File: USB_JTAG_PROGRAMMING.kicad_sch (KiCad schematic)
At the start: 85 parts, among them J16 10118194-0001LF, U3 FT2232HQ, U36 MIC5504-3.3YM5-TR, U37 93LC56BT-I/OT, U38 KC2016K12.0000C1GE00, U39 SN74LVC1T45DBVR, U40 NC7WZ07P6X, U41 NC7SZ125M5X, U42 SN74LVC1T45DBVR, U43 SN74LVC1T45DBVR, U44 SN74LVC1T45DBVR, U45 SN74LVC1T45DBVR, U46 NC7WZ126K8X, U47 NC7WZ126K8X

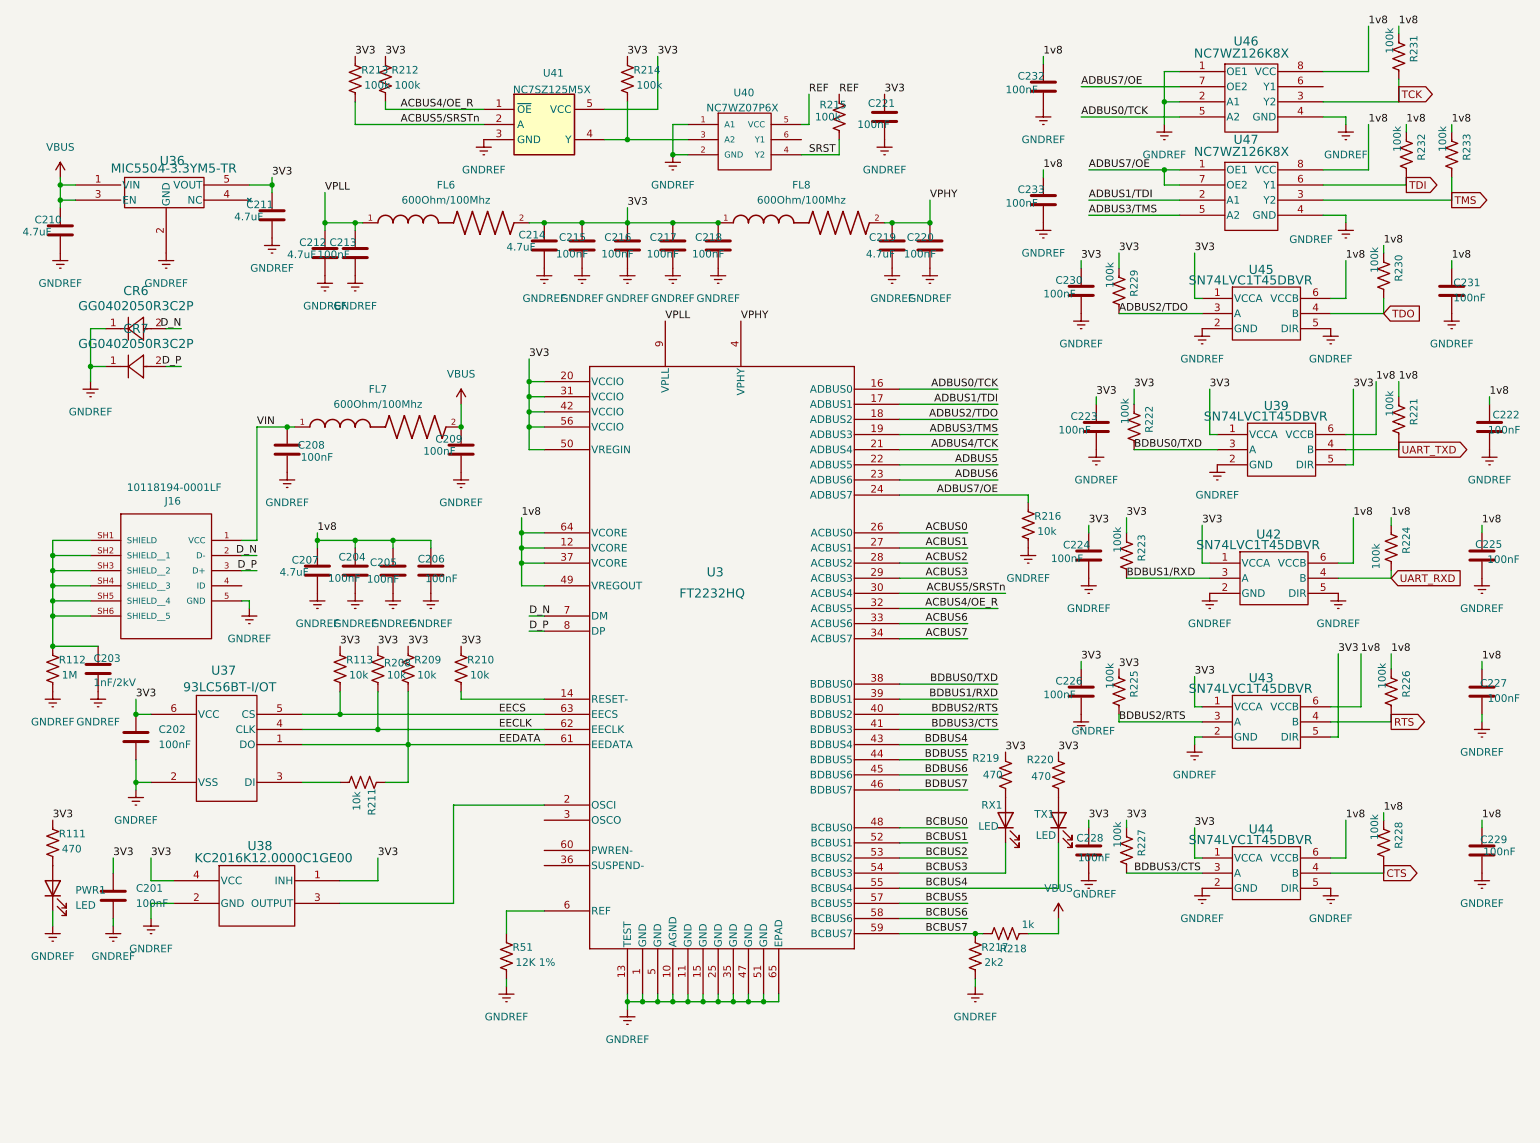
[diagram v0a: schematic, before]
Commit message: Layout update
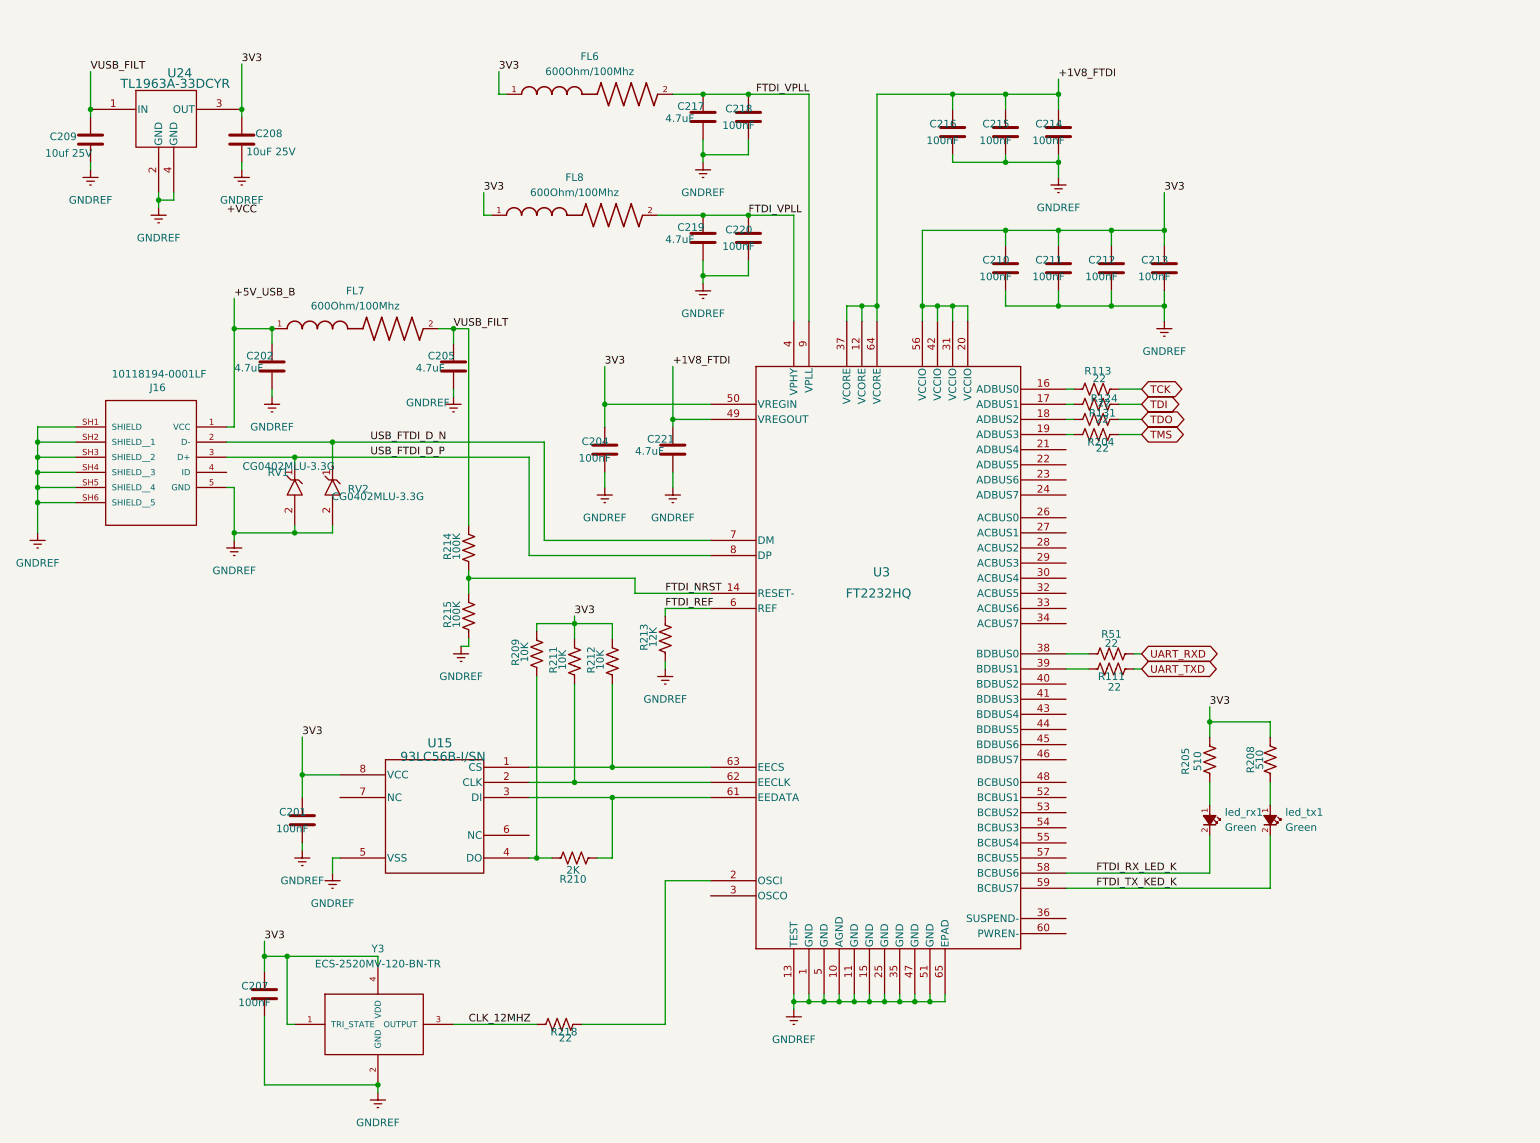
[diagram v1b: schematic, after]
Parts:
- removed C203: 1nF/2kV, footprints:C_1210_3225Metric, symbol Device:C
- removed C206, C222, C223, C224, C225, C226, C227, C228, C229, C230, C231, C232, C233: 100nF, footprints:C_0201_0603Metric, symbol Device:C
- removed CR6, CR7: GG0402050R3C2P, footprints:CR_050R3C2P_AVX, symbol GG0402050R3C2P:GG0402050R3C2P
- removed PWR1, RX1, TX1: LED, footprints:LED_0402_1005Metric, symbol Device:LED
- removed R112: 1M, footprints:R_0402, symbol Device:R_US
- removed R216: 10k, footprints:R_0402, symbol Device:R_US
- removed R217: 2k2, footprints:R_0402, symbol Device:R_US
- removed R219, R220: 470, footprints:R_0402, symbol Device:R_US
- removed R221, R222, R223, R224, R225, R226, R227, R228, R229, R230, R231, R232, R233: 100k, footprints:R_0402, symbol Device:R_US
- removed U36: MIC5504-3.3YM5-TR, footprints:SOT-23-5_MC_MCH, symbol MIC5504_3_3YM5_TR:MIC5504-3.3YM5-TR
- removed U37: 93LC56BT-I/OT, footprints:SOT-23-6_MC_MCH, symbol 93LC56BT_I_OT:93LC56BT-I_OT
- removed U38: KC2016K12.0000C1GE00, footprints:KC2016K_KYO, symbol KC2016K12-0000C1GE00:KC2016K12.0000C1GE00
- removed U39, U42, U43, U44, U45: SN74LVC1T45DBVR, footprints:DBV0006A_L, symbol SN74LVC1T45DBVR:SN74LVC1T45DBVR
- removed U40: NC7WZ07P6X, footprints:NC7WZ07P6X, symbol NC7WZ07P6X:NC7WZ07P6X
- removed U41: NC7SZ125M5X, footprints:SC-74A_318BQ_ONS, symbol 74xGxx:NC7SZ125M5X
- removed U46, U47: NC7WZ126K8X, footprints:US8-8_2P1X2P4_ONS, symbol NC7WZ126:NC7WZ126K8X
- added R124, R131, R204: 22, footprints:R_0201_0603Metric, symbol Device:R_US
- added R205: 510, footprints:R_0201_0603Metric, symbol Device:R_US
- added RV1, RV2: CG0402MLU-3.3G, footprints:VARC1005X41N, symbol CG0402MLU-3_3G:CG0402MLU-3.3G
- added U15: 93LC56B-I/SN, footprints:SOIC8-N_MC_MCH, symbol 93LC56B-I-SN:93LC56B-I_SN
- added U24: TL1963A-33DCYR, footprints:DCY4_TEX, symbol TL1963A-33DCYR:TL1963A-33DCYR
- added Y3: ECS-2520MV-120-BN-TR, footprints:OSCCC250X200X90N, symbol ECS-2520MV-120-BN-TR:ECS-2520MV-120-BN-TR
- added led_rx1, led_tx1: Green, footprints:LED_0402_1005Metric, symbol Aquiot:LED
- C202, C205, C217, C221: value 100nF -> 4.7uF; footprint footprints:C_0201_0603Metric -> footprints:C_0402; LCSC PN c1525 -> c23733
- C207, C210, C211, C212, C214: value 4.7uF -> 100nF; footprint footprints:C_0402 -> footprints:C_0201_0603Metric; LCSC PN c23733 -> c1525
- C208: value 100nF -> 10uF 25V; footprint footprints:C_0201_0603Metric -> footprints:C_0402; LCSC PN c1525 -> c23733
- C209: value 100nF -> 10uf 25V; footprint footprints:C_0201_0603Metric -> footprints:C_0402; LCSC PN c1525 -> c23733
- R111: value 470 -> 22; footprint footprints:R_0402 -> footprints:R_0201_0603Metric; LCSC PN C114877 -> (none)
- R113: value 10k -> 22; footprint footprints:R_0402 -> footprints:R_0201_0603Metric; LCSC PN C60490 -> (none)
- R208: value 10k -> 510; footprint footprints:R_0402 -> footprints:R_0201_0603Metric; LCSC PN C60490 -> (none)
- R209, R211: value 10k -> 10K; footprint footprints:R_0402 -> footprints:R_0201_0603Metric; LCSC PN C60490 -> (none)
- R210: value 10k -> 2K; footprint footprints:R_0402 -> footprints:R_0201_0603Metric; LCSC PN C60490 -> (none)
- R212: value 100k -> 10K; footprint footprints:R_0402 -> footprints:R_0201_0603Metric; LCSC PN C60491 -> (none)
- R213: value 100k -> 12K; footprint footprints:R_0402 -> footprints:R_0201_0603Metric; LCSC PN C60491 -> (none)
- R214, R215: value 100k -> 100K; footprint footprints:R_0402 -> footprints:R_0201_0603Metric; LCSC PN C60491 -> (none)
- R218: value 1k -> 22; footprint footprints:R_0402 -> footprints:R_0201_0603Metric; LCSC PN c106235 -> (none)
- R51: value 12K 1% -> 22; footprint footprints:R_0402 -> footprints:R_0201_0603Metric; LCSC PN C114760 -> (none)
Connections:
- net BDBUS0/TXD is gone; now on an unnamed net: U3.38 (BDBUS0)
- net REF is gone; now on net GNDREF: R215.1
- net 3V3: now also C204.1, C207.1, C208.1, C210.1, C212.1, C213.1, FL6.1, R208.2, R209.2, R211.2, R212.2, R205.2, U15.8 (VCC), U24.3 (OUT), Y3.1 (TRI_STATE), Y3.4 (VDD); no longer C202.1, C214.1, C215.1, C216.1, C217.1, C218.1, C221.1, FL6.2, R111.1, R113.1, R208.1, R209.1, R210.1, R212.1, R213.1, R214.1
- net GNDREF: now also J16.SH1 (SHIELD), J16.SH2 (SHIELD__1), J16.SH3 (SHIELD__2), J16.SH4 (SHIELD__3), J16.SH5 (SHIELD__4), J16.SH6 (SHIELD__5), R213.1, RV1.2, RV2.2, U15.5 (VSS), U24.2 (GND), U24.4 (GND), Y3.2 (GND); no longer R51.2
- net TCK: now also R113.2
- net TDI: now also R124.2
- net TDO: now also R131.2
- net TMS: now also R204.2
- net UART_RXD: now also R51.2
- net UART_TXD: now also R111.2
- net at R51.1: no longer U3.6 (REF)
- net at U3.2 (OSCI): now also R218.2
- net at R210.2: now also R209.1, U15.4 (DO); no longer U3.14 (RESET-)
- net VUSB_FILT: now reaches R214.2
- net VUSB_FILT: now also C205.1, C209.1, FL7.2, U24.1 (IN)
- net 1v8 renamed +1V8_FTDI
- net +1V8_FTDI: now also C214.1, C215.1, C216.1, C221.1; no longer C204.1, C205.1, C207.1
- net ACBUS0: no longer names the net of U3.26 (ACBUS0)
- net ACBUS1: no longer names the net of U3.27 (ACBUS1)
- net ACBUS2: no longer names the net of U3.28 (ACBUS2)
- net ACBUS3: no longer names the net of U3.29 (ACBUS3)
- net ACBUS4/OE_R: no longer names the net of U3.32 (ACBUS5)
- net ACBUS4/OE_R: no longer R212.2
- net ACBUS5/SRSTn: no longer names the net of U3.30 (ACBUS4)
- net ACBUS5/SRSTn: no longer R213.2
- net ACBUS6: no longer names the net of U3.33 (ACBUS6)
- net ACBUS7: no longer names the net of U3.34 (ACBUS7)
- net ADBUS0/TCK: no longer names the net of U3.16 (ADBUS0)
- net ADBUS0/TCK: now also R113.1
- net ADBUS1/TDI: no longer names the net of U3.17 (ADBUS1)
- net ADBUS1/TDI: now also R124.1
- net ADBUS2/TDO: no longer names the net of U3.18 (ADBUS2)
- net ADBUS2/TDO: now also R131.1
- net ADBUS3/TMS: no longer names the net of U3.19 (ADBUS3)
- net ADBUS3/TMS: now also R204.1
- net ADBUS4/TCK: no longer names the net of U3.21 (ADBUS4)
- net ADBUS5: no longer names the net of U3.22 (ADBUS5)
- net ADBUS6: no longer names the net of U3.23 (ADBUS6)
- net ADBUS7/OE: no longer names the net of U3.24 (ADBUS7)
- net BCBUS0: no longer names the net of U3.48 (BCBUS0)
- net BCBUS1: no longer names the net of U3.52 (BCBUS1)
- net BCBUS2: no longer names the net of U3.53 (BCBUS2)
- net BCBUS3: no longer names the net of U3.54 (BCBUS3)
- net BCBUS4: no longer names the net of U3.55 (BCBUS4)
- net BCBUS5: no longer names the net of U3.57 (BCBUS5)
- net BCBUS6 renamed FTDI_RX_LED_K
- net FTDI_RX_LED_K: now also led_rx1.2 (K)
- net BCBUS7 renamed CLK_12MHZ
- net CLK_12MHZ: now also Y3.3 (OUTPUT); no longer U3.59 (BCBUS7)
- net BDBUS1/RXD: no longer names the net of U3.39 (BDBUS1)
- net BDBUS1/RXD: now also R111.1
- net BDBUS2/RTS: no longer names the net of U3.40 (BDBUS2)
- net BDBUS3/CTS: no longer names the net of U3.41 (BDBUS3)
- net BDBUS4: no longer names the net of U3.43 (BDBUS4)
- net BDBUS5: no longer names the net of U3.44 (BDBUS5)
- net BDBUS6: no longer names the net of U3.45 (BDBUS6)
- net BDBUS7: no longer names the net of U3.46 (BDBUS7)
- net D_N renamed USB_FTDI_D_N
- net USB_FTDI_D_N: now also RV2.1
- net D_P renamed USB_FTDI_D_P
- net USB_FTDI_D_P: now also RV1.1
- net EECLK: no longer names the net of U3.62 (EECLK)
- net EECLK: now also R211.1, U15.2 (CLK); no longer R208.2
- net EECS: no longer names the net of U3.63 (EECS)
- net EECS: now also R212.1, U15.1 (CS); no longer R113.2
- removed net EEDATA: R209.2, R211.1, U3.61 (EEDATA)
- net SRST renamed FTDI_NRST
- net FTDI_NRST: now also R214.1, U3.14 (RESET-)
- removed net VBUS: C209.1, C210.1, FL7.2, R218.2
- net VIN renamed +5V_USB_B
- net +5V_USB_B: now also C202.1; no longer C208.1
- net VPHY renamed FTDI_VPLL
- net FTDI_VPLL: now also C217.1, C218.1, FL6.2, U3.9 (VPLL)
- removed net VPLL: C212.1, C213.1, FL6.1, U3.9 (VPLL)
- new net: R210.1, U15.3 (DI), U3.61 (EEDATA)
- new net: R205.1, led_rx1.1 (A)
- new net: R208.1, led_tx1.1 (A)
- new net FTDI_REF: R213.2, U3.6 (REF)
- new net FTDI_TX_KED_K: U3.59 (BCBUS7), led_tx1.2 (K)
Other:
- moved on the sheet: J16, U3
